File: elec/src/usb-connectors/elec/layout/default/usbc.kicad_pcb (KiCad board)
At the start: 2 copper layers, 3 parts

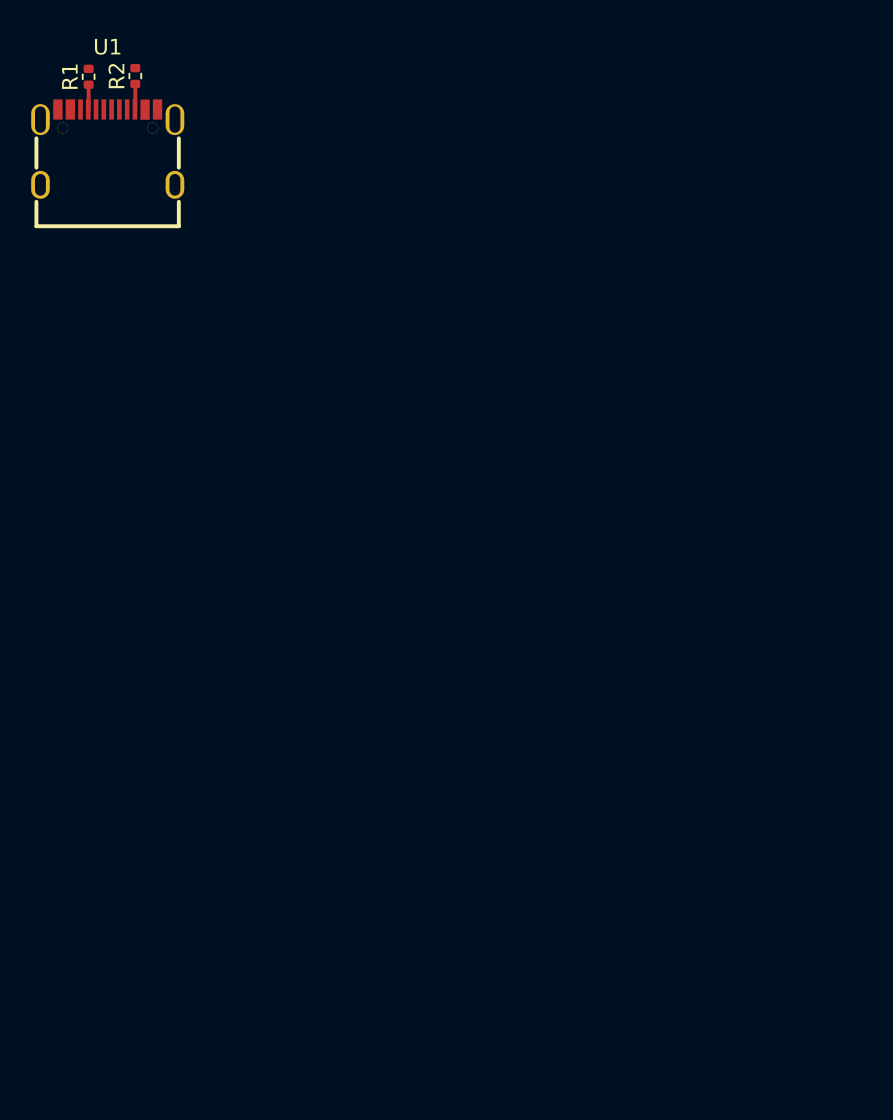
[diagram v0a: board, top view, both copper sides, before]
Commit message: fixed maybe
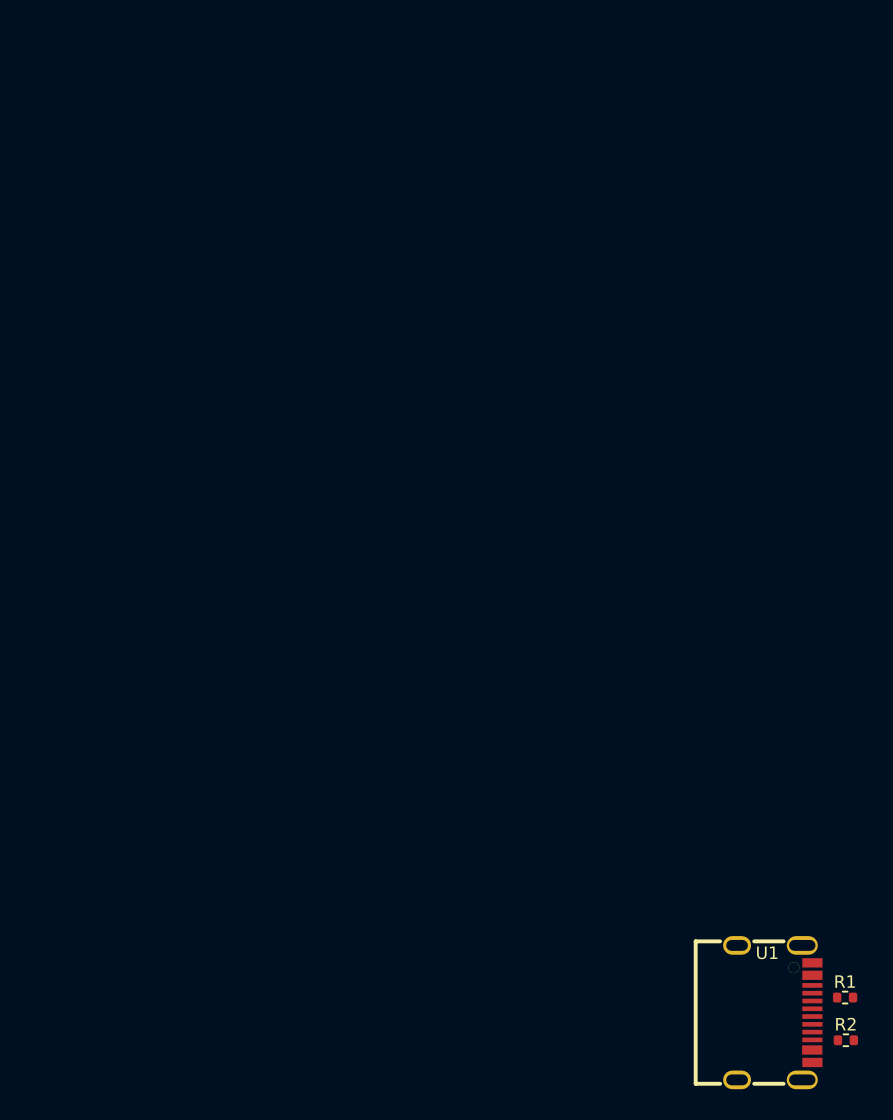
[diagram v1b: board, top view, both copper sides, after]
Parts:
- moved R2 77.0 mm to (178.0, 122.3), turned to 0 degrees
- moved R1 76.6 mm to (178.0, 119.6), turned to 0 degrees
- moved U1 70.2 mm to (173.5, 120.6), turned to -90 degrees
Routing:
- net cc2: track 1.65 -> 0.00 mm
- net cc1: track 1.60 -> 0.00 mm
